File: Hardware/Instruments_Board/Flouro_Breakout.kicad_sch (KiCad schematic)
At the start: 15 parts, among them J1 RJ45_LED_Shielded, U1 Teensy4.1_DEV-16771, U2 3V3 OKI

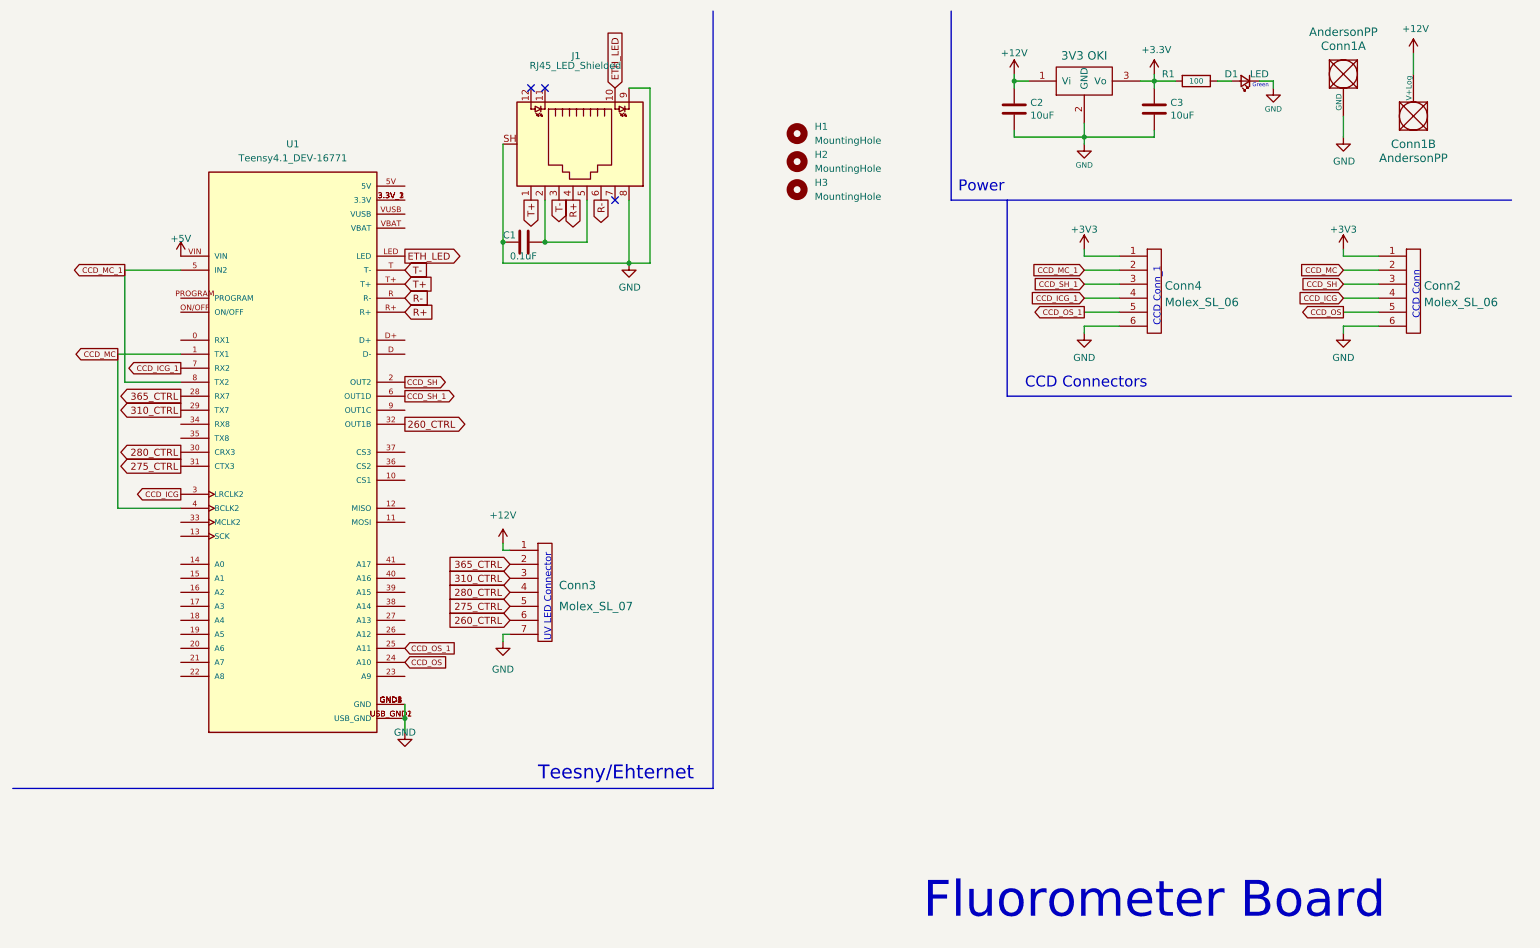
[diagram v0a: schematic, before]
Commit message: finished fluoro breakout
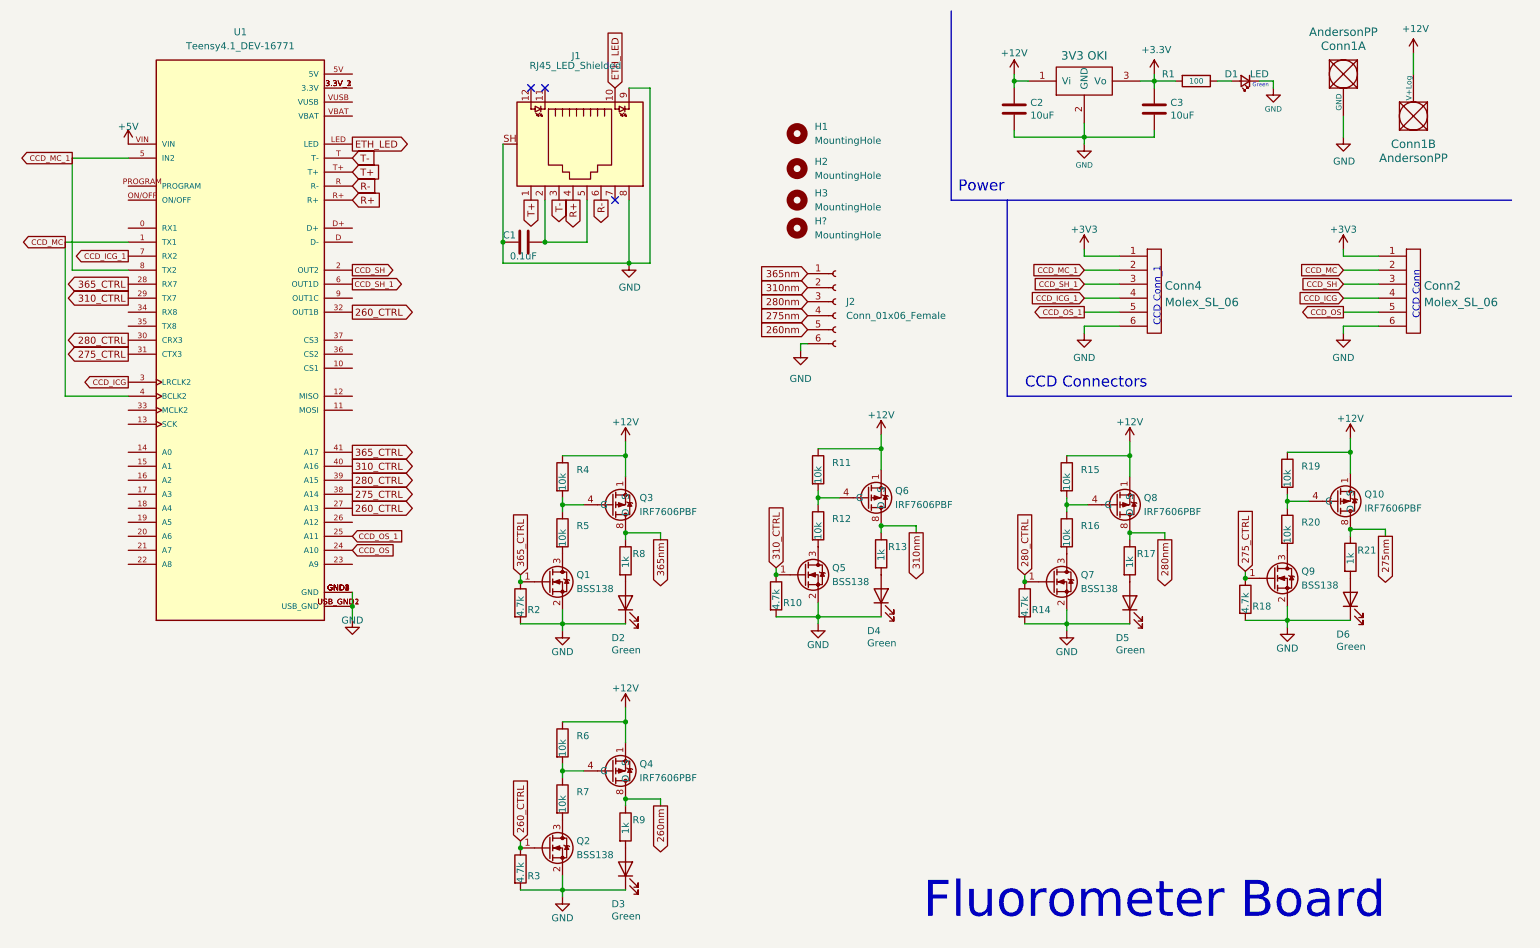
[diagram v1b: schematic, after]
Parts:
- removed Conn3: Molex_SL_07, MRDT_Connectors:MOLEX_SL_07_Vertical, symbol MRDT_Connectors:Molex_SL_07
- added D2, D3, D4, D5, D6: Green, LED_SMD:LED_0603_1608Metric_Pad1.05x0.95mm_HandSolder, symbol Device:LED
- added H?: MountingHole, MRDT_Drill_Holes:4_40_Hole_Corner, symbol Mechanical:MountingHole
- added J2: Conn_01x06_Female, Connector_Molex:Molex_SL_171971-0006_1x06_P2.54mm_Vertical, symbol Connector:Conn_01x06_Female
- added Q1, Q2, Q5, Q7, Q9: BSS138, Package_TO_SOT_SMD:SOT-23, symbol Transistor_FET:BSS138
- added Q10, Q3, Q4, Q6, Q8: IRF7606PBF, Package_SO:SOP-8_3.9x4.9mm_P1.27mm, symbol Transistor_FET:IRF7606PBF
- added R10, R14, R18, R2, R3: 4.7k, Resistor_SMD:R_0603_1608Metric_Pad0.98x0.95mm_HandSolder, symbol Device:R
- added R11, R12, R15, R16, R19, R20, R4, R5, R6, R7: 10k, Resistor_SMD:R_0603_1608Metric_Pad0.98x0.95mm_HandSolder, symbol Device:R
- added R13, R17, R21, R8, R9: 1k, Resistor_SMD:R_0603_1608Metric_Pad0.98x0.95mm_HandSolder, symbol Device:R
- H1, H2, H3: footprint MountingHole:MountingHole_3.2mm_M3 -> MRDT_Drill_Holes:4_40_Hole_Corner
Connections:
- net +12V: now also Q10.1 (S), Q10.2 (S), Q10.3 (S), Q3.1 (S), Q3.2 (S), Q3.3 (S), Q4.1 (S), Q4.2 (S), Q4.3 (S), Q6.1 (S), Q6.2 (S), Q6.3 (S), Q8.1 (S), Q8.2 (S), Q8.3 (S), R11.1, R15.1, R19.1, R4.1, R6.1
- net 260_CTRL: now also U1.27 (A13), Q2.1 (G), R3.1
- net 275_CTRL: now also U1.38 (A14), Q9.1 (G), R18.1
- net 280_CTRL: now also U1.39 (A15), Q7.1 (G), R14.1
- net 310_CTRL: now also U1.40 (A16), Q5.1 (G), R10.1
- net 365_CTRL: now also U1.41 (A17), Q1.1 (G), R2.1
- net GND: now also D2.1 (K), D3.1 (K), D4.1 (K), D5.1 (K), D6.1 (K), J2.6 (Pin_6), Q1.2 (S), Q2.2 (S), Q5.2 (S), Q7.2 (S), Q9.2 (S), R10.2, R14.2, R18.2, R2.2, R3.2
- new net: Q4.4 (G), R6.2, R7.1
- new net: Q6.4 (G), R11.2, R12.1
- new net: D5.2 (A), R17.2
- new net: D3.2 (A), R9.2
- new net: Q9.3 (D), R20.2
- new net: Q3.4 (G), R4.2, R5.1
- new net: Q10.4 (G), R19.2, R20.1
- new net: D2.2 (A), R8.2
- new net: Q1.3 (D), R5.2
- new net: Q8.4 (G), R15.2, R16.1
- new net: Q5.3 (D), R12.2
- new net: Q2.3 (D), R7.2
- new net: D4.2 (A), R13.2
- new net: D6.2 (A), R21.2
- new net: Q7.3 (D), R16.2
- new net 260nm: J2.5 (Pin_5), Q4.5 (D), Q4.6 (D), Q4.7 (D), Q4.8 (D), R9.1
- new net 275nm: J2.4 (Pin_4), Q10.5 (D), Q10.6 (D), Q10.7 (D), Q10.8 (D), R21.1
- new net 280nm: J2.3 (Pin_3), Q8.5 (D), Q8.6 (D), Q8.7 (D), Q8.8 (D), R17.1
- new net 310nm: J2.2 (Pin_2), Q6.5 (D), Q6.6 (D), Q6.7 (D), Q6.8 (D), R13.1
- new net 365nm: J2.1 (Pin_1), Q3.5 (D), Q3.6 (D), Q3.7 (D), Q3.8 (D), R8.1
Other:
- note removed: "Teesny/Ehternet"
- note removed: "UV LED Connector"
- moved on the sheet: U1
